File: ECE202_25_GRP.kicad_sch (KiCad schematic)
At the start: 9 parts, among them K1 JQC-3FF-009-1Z, K2 JQC-3FF-009-1Z, K3 JQC-3FF-009-1Z, K4 JQC-3FF-009-1Z, U1 NE555P

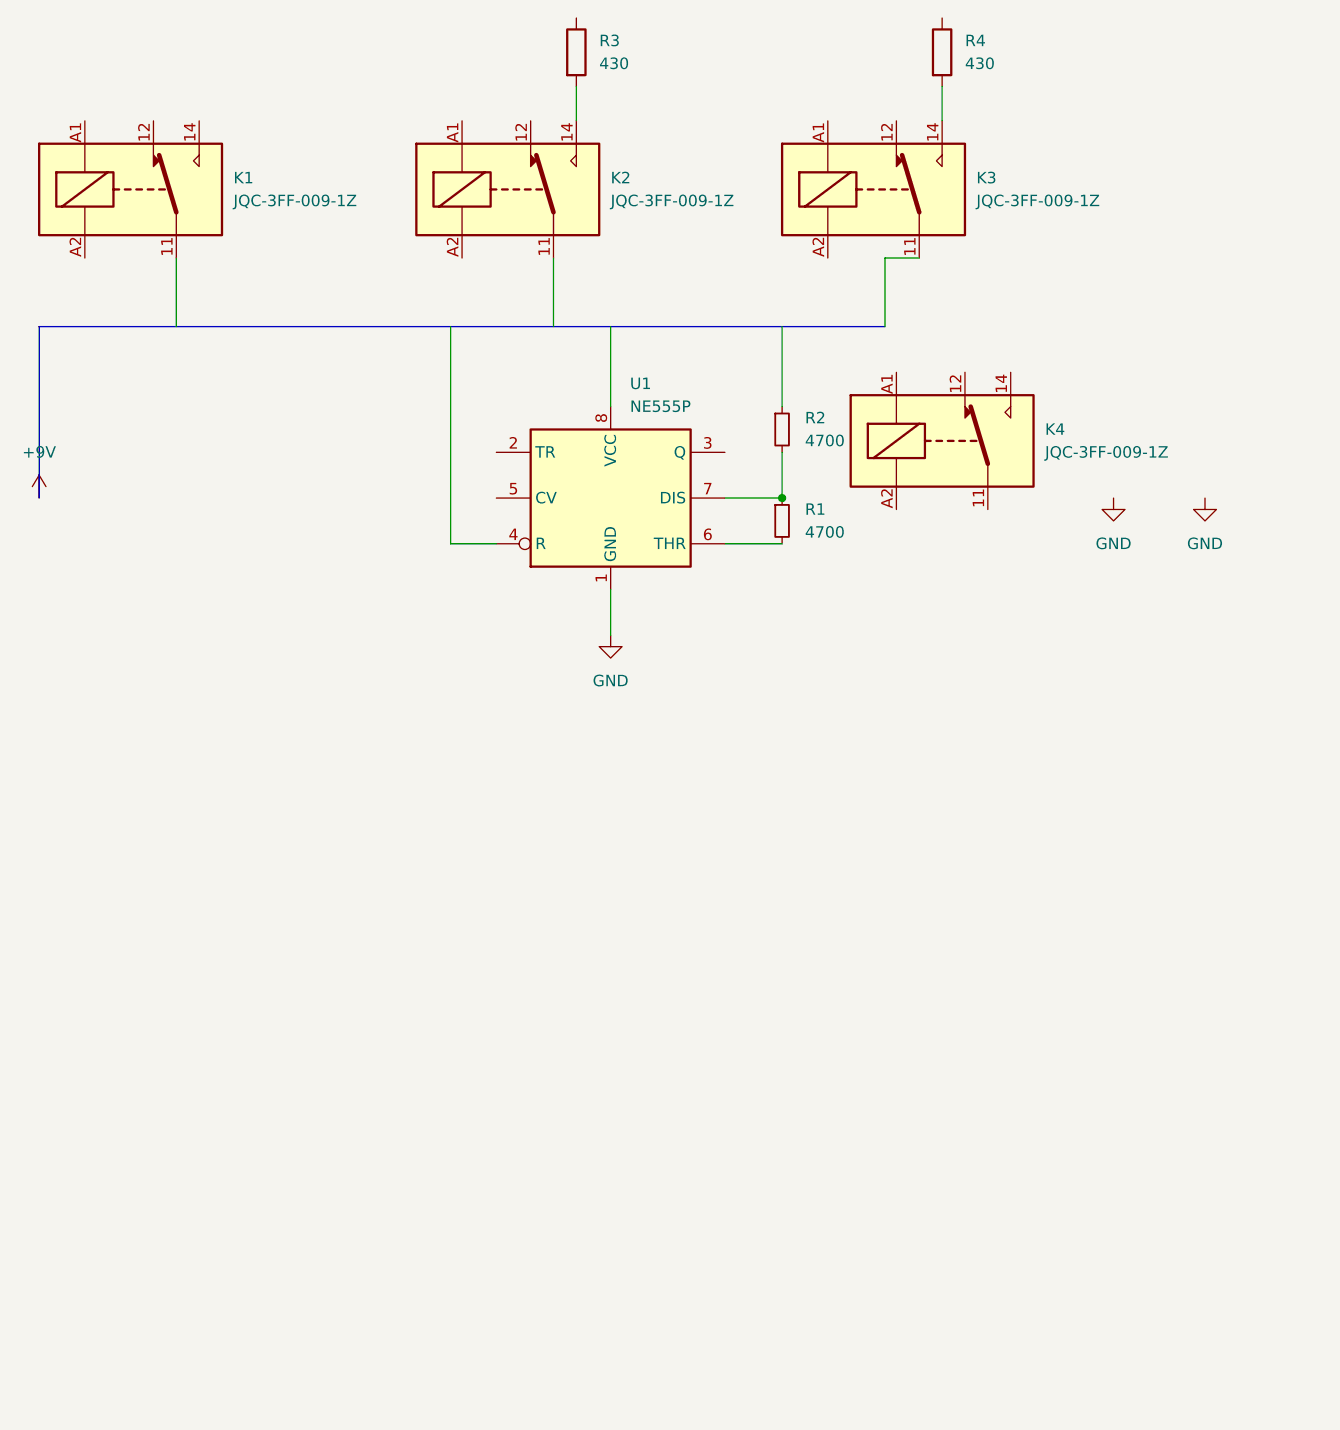
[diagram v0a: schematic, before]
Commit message: Finished V1 of schematic
Screen shot in new images folder
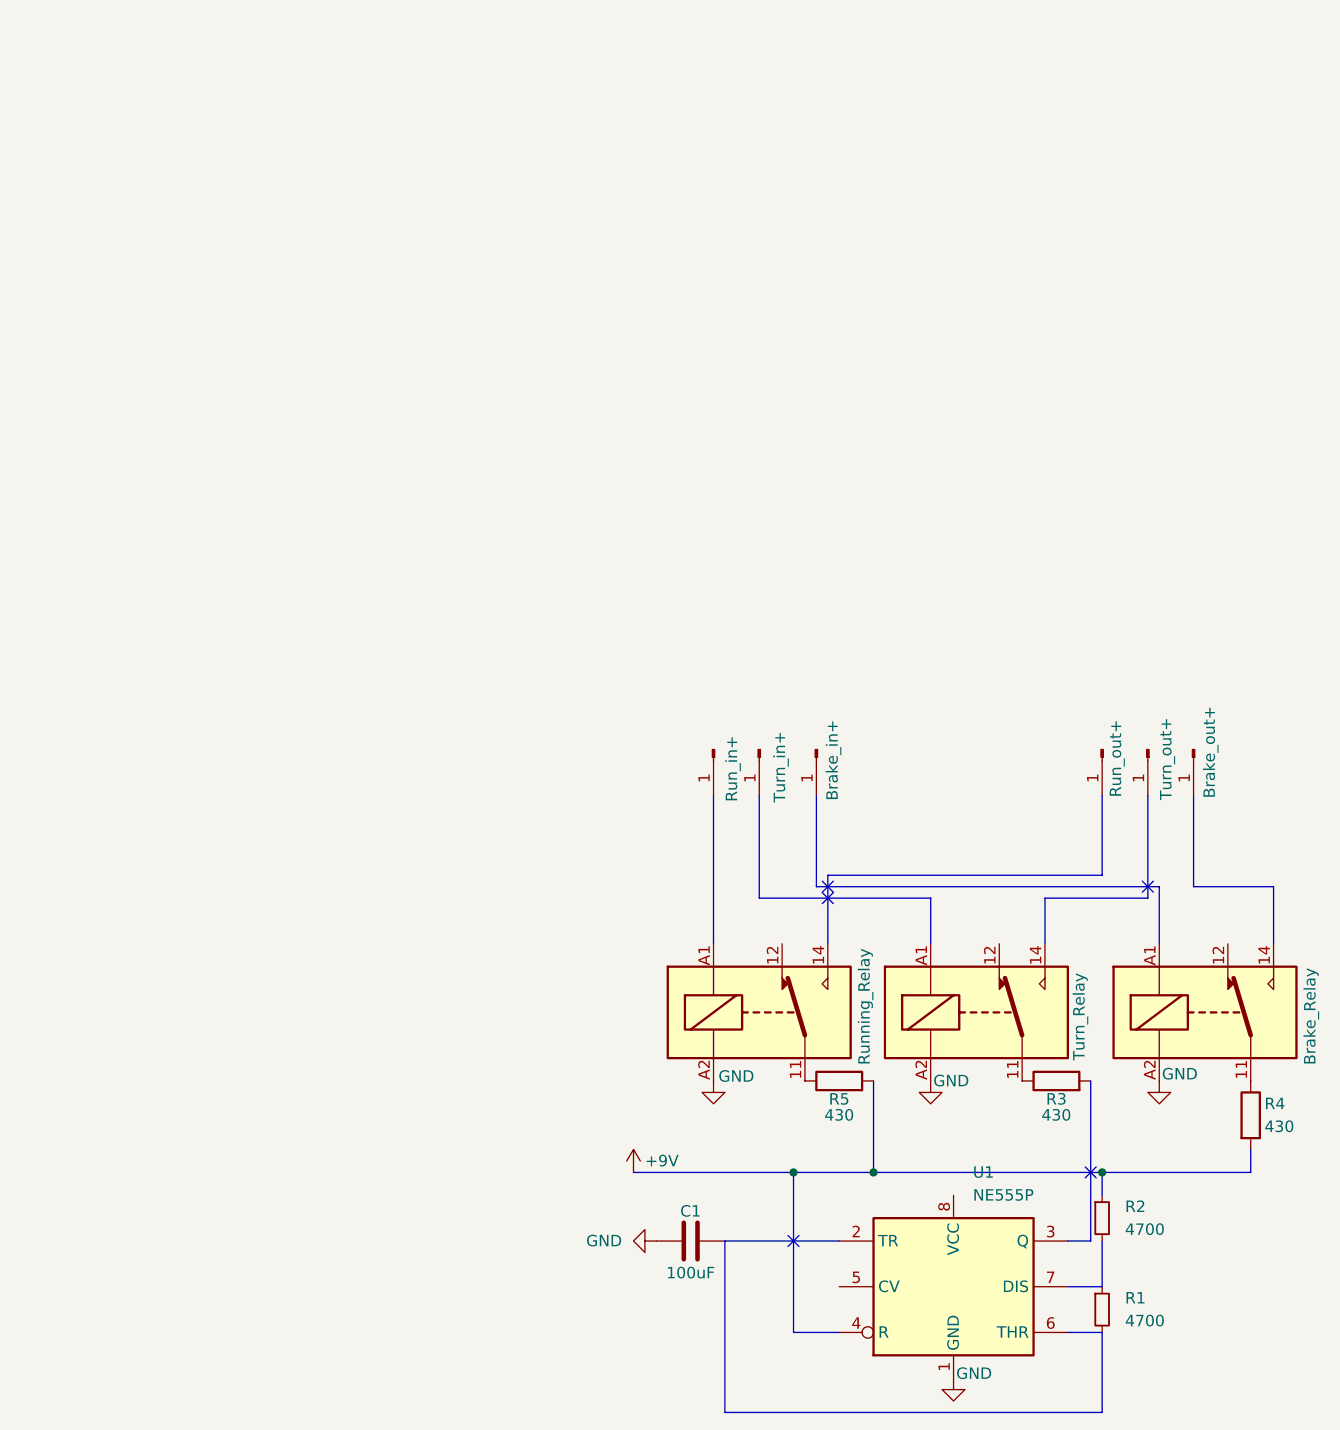
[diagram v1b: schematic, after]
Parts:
- removed K4: JQC-3FF-009-1Z, Relay_THT:Relay_SPDT_Hongfa_JQC-3FF_0XX-1Z, symbol Relay:JQC-3FF-009-1Z
- added C1: 100uF, symbol Device:C
- added J1: Run_in+, symbol Connector:Conn_01x01_Pin
- added J2: Brake_in+, symbol Connector:Conn_01x01_Pin
- added J3: Turn_in+, symbol Connector:Conn_01x01_Pin
- added J4: Run_out+, symbol Connector:Conn_01x01_Pin
- added J5: Brake_out+, symbol Connector:Conn_01x01_Pin
- added J6: Turn_out+, symbol Connector:Conn_01x01_Pin
- added R5: 430, symbol Device:R
- K1: value JQC-3FF-009-1Z -> Running_Relay
- K2: value JQC-3FF-009-1Z -> Turn_Relay
- K3: value JQC-3FF-009-1Z -> Brake_Relay
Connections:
- net GND: now also K1.A2, K2.A2, K3.A2, C1.1
- net at R4.1: now also K3.11
- net at R4.2: no longer K3.14
- net at K2.11: now also R3.1
- net at K2.14: no longer R3.2
- net at K1.11: now also R5.1
- net at U1.6 (THR): no longer R1.2
- now unconnected: R1.1, R2.2, U1.7 (DIS)
- no-connect marks 0 -> 5
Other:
- company: (none) -> HME Designs
- title: (none) -> LED Automotive Lighting Main PCB
- moved on the sheet: R1, R2, R3, R4, U1
